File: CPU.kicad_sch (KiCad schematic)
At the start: 153 parts, among them P1 Conn_02x36_Top_Bottom, P2 Conn_02x13_Top_Bottom, P3 Conn_02x13_Top_Bottom, P4 Conn_02x08_Counter_Clockwise, P5 Conn_02x25_Counter_Clockwise, P6 Conn_02x25_Counter_Clockwise, P7 Conn_02x07_Counter_Clockwise

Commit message: partial memory board
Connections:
- net Sys.PA_{14} is gone; now on net Sys.~{PA_{14}}: P1.19 (Pin_19)
- net Sys.~{Parity}: now reaches P1.29 (Pin_29), U_A13.11
- net Sys.~{INTACK}: now reaches P1.65 (Pin_65), U_A14.11
- net Sys.~{PA_{14}}: now reaches U_A9.12 (BUS2)
- net A13D_a renamed ParitySelect
- net DMA_P2_12 renamed DMAINTRequest
- net E10_8_F14_2 renamed ~{DMAInterrupt}
- net Sys.A_{0} renamed Sys.~{A_{0}}
- net Sys.A_{10} renamed Sys.~{A_{10}}
- net Sys.A_{1} renamed Sys.~{A_{1}}
- net Sys.A_{2} renamed Sys.~{A_{2}}
- net Sys.A_{3} renamed Sys.~{A_{3}}
- net Sys.A_{4} renamed Sys.~{A_{4}}
- net Sys.A_{5} renamed Sys.~{A_{5}}
- net Sys.A_{6} renamed Sys.~{A_{6}}
- net Sys.A_{7} renamed Sys.~{A_{7}}
- net Sys.A_{8} renamed Sys.~{A_{8}}
- net Sys.A_{9} renamed Sys.~{A_{9}}
- net Sys.CA_{15} renamed Sys.~{CA_{15}}
- net Sys.D_{0} renamed Sys.~{D_{0}}
- net Sys.D_{1} renamed Sys.~{D_{1}}
- net Sys.D_{2} renamed Sys.~{D_{2}}
- net Sys.D_{3} renamed Sys.~{D_{3}}
- net Sys.D_{4} renamed Sys.~{D_{4}}
- net Sys.D_{5} renamed Sys.~{D_{5}}
- net Sys.D_{6} renamed Sys.~{D_{6}}
- net Sys.D_{7} renamed Sys.~{D_{7}}
- net Sys.E_{63} renamed Sys.~{INTREQ}
- net Sys.E_{64} renamed Sys.~{MemFault}
- net Sys.INR0 renamed Sys.~{INR0}
- net Sys.INR1 renamed Sys.~{INR1}
- net Sys.INR2 renamed Sys.~{INR2}
- net Sys.INR3 renamed Sys.~{INR3}
- net Sys.PA_{12} renamed Sys.~{PA_{12}}
- net Sys.PA_{13} renamed Sys.~{PA_{13}}
- net Sys.PA_{15} renamed Sys.~{PA_{15}}
- net Sys.PA_{16} renamed Sys.~{PA_{16}}
- net Sys.PA_{17} renamed Sys.~{PA_{17}}
- net ~{AND_SysE_{64}} renamed MemFault_EN
- net ~{DMA_P2_12} renamed ~{DMAINTRequest}
- net ~{DMA_P2_13} renamed ~{DMARequest}
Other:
- note added: "F14D = LOW IF (SW_H=open AND DMA Interrupt) typically HIGH"
- note added: "Sys.~{INR3}"
- note removed: "BusCtl Func: DMA?"
- note removed: "F14D = LOW IF (SW_H=open AND DMA_INT_Request?) typically HIGH"
- note removed: "INT ACK ?"
- moved on the sheet: U_A13D, U_A14D

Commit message: lots of layout and DMA labels, weeee
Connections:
- net MW.D3_{3} is gone; now on net TODO_D3_{3}: U_L5.9 (Q3)
- net SEQ.S_{0} is gone; now on net SEQ.SH_{0}: U_J7.16 (S_{0}), U_L9.10 (S_{0})
- net ~{H14_OE} is gone; now on net TODO_A8_7: U_D5.12 (Q4), U_H14.1 (OEa)
- net DataF.D_{0}: now also U_K7.5 (R_{0})
- net DataF.D_{1}: now also U_K7.4 (R_{1})
- net DataF.D_{2}: now also U_K7.3 (R_{2})
- net FP.~{ABT}: now also R1.2, U_M14.7 (O1b); no longer P3.16 (Pin_16), R1.1
- net GND: now also DSW1.10, DSW1.11, DSW1.12, DSW1.13, DSW1.14, DSW1.15, DSW1.16, DSW1.9, U_M14.19 (OEb)
- net MW.C4_{0}: now also U_J6.5, U_K6.4
- net MW.F1_{7}: now also U_K9.7 (~{E})
- net ~{DataRDLatch}: now also U_B15.3 (C)
- net DMA.~{StartCycle}: now reaches P2.10 (Pin_10), R4.3 (R2), U_M8.8 (I3a)
- net TODO_D3_{3}: now reaches U_L6.4
- net ~{RTC_INT_Reset}: now reaches U_M13.10 (Q5), U_M9.13 (~{R})
- net DMA.~{AddressControl}: now reaches P2.2 (Pin_2), U_M8.9 (O0b)
- net DMA.~{Enable}: now reaches P2.6 (Pin_6), U_M8.3 (O3b)
- net DMA.~{Enable}: no longer U_M8.16 (O1a)
- net DMA.~{BusWriteOE}: now reaches P2.9 (Pin_9), U_M10.8
- net SEQ.SH_{0}: now reaches U_K6.3
- net AddrHToSys renamed ~{AddrHToSys}
- net C15_~{PE}: no longer names the net of U_B11.6, U_C10.3, U_C15.9 (~{PE}), U_D6.10 (I1c)
- net DMAWrite renamed DMA.Write
- net FPC_P3_9 renamed ~{ResetFlag}
- net J7_S_{1} renamed SEQ.S1_{1}
- net K9_In4 renamed CondRegOrPageOut
- net K9_In5 renamed CondDMARequest
- net K9_In6 renamed CondMemFault
- net K9_In7 renamed CondMultiINT
- net L9_S_{1} renamed SEQ.S2_{1}
- net Sys.~{Parity} renamed Sys.~{ParityTest}
- net ~{DMAINTRequest} renamed DMA.~{INTRequest}
- net ~{DMARequest} renamed DMA.~{Request}
- net ~{FPC_P3_15} renamed ~{FPC_SW_4}
- new net: P3.16 (Pin_16), R1.1
- new net DMA.~{End}: U_M8.16 (O1a)
- no-connect marks 54 -> 60
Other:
- note added: "(IN)"
- note added: "(OUT)"
- note added: "+5"
- note added: "ABT"
- note added: "ABT LED"
- note added: "B8A output goes LOW when all are HIGH: AND PA_{17} AND PA_{16} AND PA_{15}^{(?)} AND PA_{14},PA_{13} AND PA_{11} AND PTR.Q_{7} * ignores PA_{12} * PTR.Q_{7} (high bit) has extra memory functions attached (likely page control and MMIO selection) * this would select (ignoring the page bit): ** 0x3f8nn to 0x3ffnn ** ** 0x3e8nn to 0x3efnn **"
- note added: "Edge Top 11 (aka pin47 or Sys.~{APRE}) is OC and follows the output of B7A (pulls LOW when REGFILE addressed) ~{APRE} is not read by the CPU, it's used by memory/cards"
- note added: "GND"
- note added: "GND?"
- note added: "HALT"
- note added: "Holds at zero while no bus cycle Counts up from zero during a cycle Stops at 15 and asserts Sys.~{DRDY}"
- note added: "INR is not in order"
- note added: "Line Clock"
- note added: "MAP0"
- note added: "MAP1"
- note added: "MAP2"
- note added: "RUN"
- note added: "RUN/~{HALT}"
- note added: "SS 2 (OPSYS)"
- note added: "SS 4 (R/F)"
- note added: "SW_M SW_O probably need pull R"
- note added: "SW_O"
- note added: "See E6 (K12.4?)"
- note added: "SysCtl.0 DMA"
- note added: "SysCtl.1 DMA"
- note added: "TODO M8.3,16 to P2"
- note added: "This loads the Condition Register (through extra logic?)"
- note added: "Write/~{Read}"
- note added: "these 3 pins drive the register file index their order does not matter after this point"
- note added: "this half should be GND?"
- note removed: "B8A output goes LOW when all are HIGH: AND PA_{17} AND PA_{16} AND PA_{15}^{(?)} AND PA_{14},PA_{13} AND PA_{11} AND PTR.Q_{7} * ignores PA_{12} * PTR.Q_{7} (high bit) has extra memory functions attached (likely page control and MMIO selection) * this would select (ignoring the high bit): ** 0x3f8nn to 0x3ffnn ** ** 0x3e8nn to 0x3efnn **"
- note removed: "Counts up from zero (sync-load) Stops at 15"
- note removed: "Edge Top 11 (aka pin47 or Sys.~{APRE}) is OC and follows the output of B7A (pulls LOW when REGFILE addressed)"
- note removed: "Sys.~{INR3}"
- note removed: "does M8.12 float? or is the cross connect wrong?"
- note removed: "these three pins drive the register file index their order does not matter after this point"
- moved on the sheet: BODGE1, C39, CR1, P1, P2, P3, P7, R1, R15, R17, R2, R3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

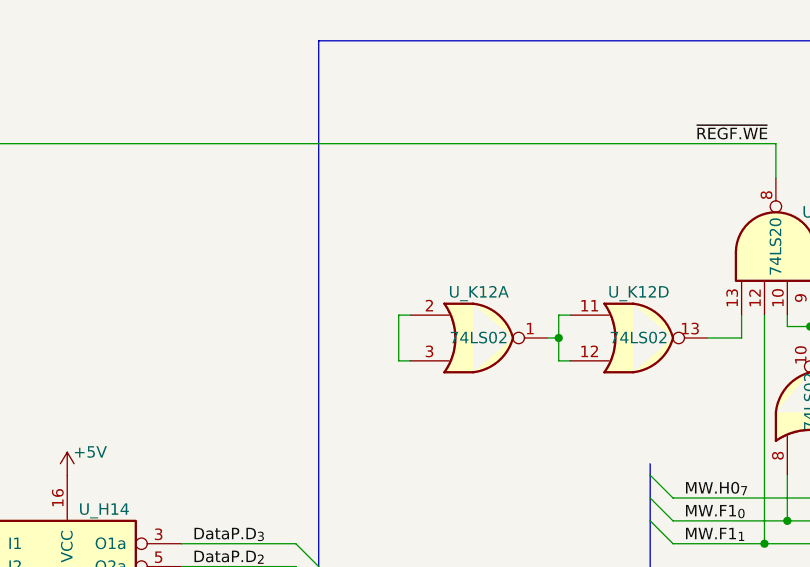
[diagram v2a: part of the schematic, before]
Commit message: an important guess?
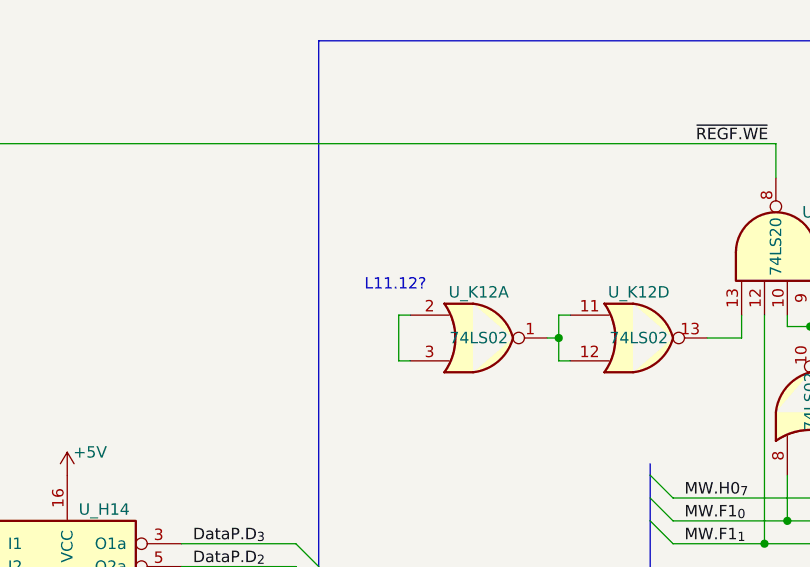
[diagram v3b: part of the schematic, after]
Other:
- note added: "L11.12?"
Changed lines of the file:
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@@
+    (effects (font (size 1.27 1.27)) (justify left bottom))
+  )
+  (text "L11.12?" (at 589.28 114.3 0)
     (effects (font (size 1.27 1.27)) (justify left bottom))
   )

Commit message: all the pins!? and another ERC pass
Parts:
- removed BODGE1: Jumper_2_Bridged, symbol Jumper:Jumper_2_Bridged
- added P10, P8: Conn_02x08_Counter_Clockwise, Package_DIP:DIP-16_W7.62mm_Socket, symbol Connector_Generic:Conn_02x08_Counter_Clockwise
- added unit 3 of U_A1
- added unit 5 of U_A13
- added unit 5 of U_A14
- added unit 7 of U_A15
- added unit 5 of U_A2
- added unit 7 of U_A3
- added unit 4 of U_B11
- added unit 5 of U_B12
- added unit 3 of U_B15
- added unit 2 of U_B7
- added unit 2 of U_B8
- added unit 7 of U_C10
- added unit 5 of U_C7
- added unit 7 of U_C8
- added unit 5 of U_D10
- added unit 5 of U_D12
- added unit 3 of U_D2
- added unit 3 of U_D8
- added unit 4 of U_E10
- added unit 4 of U_E11
- added unit 7 of U_E12
- added unit 7 of U_E14
- added unit 3 of U_E15
- added unit 5 of U_E8
- added unit 3 of U_F12
- added unit 5 of U_F14
- added unit 3 of U_H13
- added unit 7 of U_J6
- added unit 5 of U_K10
- added unit 5 of U_K12
- added unit 5 of U_K6
- added unit 3 of U_L10
- added unit 3 of U_L13
- added unit 5 of U_L14
- added unit 5 of U_L6
- added unit 5 of U_M10
- added unit 3 of U_M9
- C39: footprint (none) -> Capacitor_THT:CP_Axial_L20.0mm_D10.0mm_P26.00mm_Horizontal
- CR1: footprint (none) -> Diode_THT:D_A-405_P10.16mm_Horizontal
- DSW1: footprint (none) -> Package_DIP:DIP-16_W7.62mm_Socket_LongPads
- JP1: footprint (none) -> Connector_PinHeader_2.54mm:PinHeader_1x03_P2.54mm_Vertical
- P1: footprint (none) -> Connector_PCBEdge:BUS_EE200
- P2, P3: footprint (none) -> Connector_IDC:IDC-Header_2x13_P2.54mm_Horizontal
- P4: footprint (none) -> Package_DIP:DIP-16_W7.62mm_Socket
- P5, P6: footprint (none) -> Connector_PinHeader_2.54mm:PinHeader_2x25_P2.54mm_Vertical; symbol Connector_Generic:Conn_02x25_Counter_Clockwise -> Connector_Generic:Conn_02x25_Odd_Even
- P7: footprint (none) -> Package_DIP:DIP-14_W7.62mm_Socket
- R1, R10, R11, R12, R13, R14, R15, R17, R18, R19, R2, R3, R5, R6, R8, R9: footprint (none) -> Resistor_THT:R_Axial_DIN0207_L6.3mm_D2.5mm_P10.16mm_Horizontal
- U_A1, U_A13, U_A14, U_A15, U_A2, U_A3, U_B11, U_B12, U_B15, U_B7, U_B8, U_C10, U_C7, U_C8, U_D10, U_D12, U_D8, U_E10, U_E11, U_E12, U_E14, U_E15, U_E8, U_F12, U_F14, U_H13, U_J6, U_K10, U_K12, U_K6, U_L10, U_L14, U_L6, U_M10, U_M9: footprint (none) -> Package_DIP:DIP-14_W7.62mm
- U_A10, U_A4, U_A5, U_A6, U_A8, U_A9, U_B1, U_B2, U_B3, U_B4, U_B5, U_B6, U_C1, U_C11, U_C12, U_C14, U_C15, U_C2, U_C3, U_C4, U_C5, U_C6, U_D11, U_D2, U_D3, U_D4, U_D5, U_D6, U_D7, U_D9, U_E5, U_E6, U_E7, U_F11, U_F13, U_F6, U_H11, U_H12, U_H14, U_H6, U_J10, U_J11, U_J12, U_J13, U_J9, U_K11, U_K13, U_K9, U_L11, U_L13, U_M12, U_M13: footprint (none) -> Package_DIP:DIP-16_W7.62mm
- U_A11, U_A12, U_A7, U_B13, U_C13, U_C9, U_D13, U_F5, U_H5, U_J5, U_K5, U_L5, U_M14, U_M15, U_M5, U_M6, U_M7, U_M8: footprint (none) -> Package_DIP:DIP-20_W7.62mm
- U_B10, U_B9, U_D14, U_D15: footprint (none) -> Package_DIP:DIP-22_W7.62mm_Socket
- U_J7, U_K7: footprint (none) -> Package_DIP:DIP-28_W15.24mm_Socket
- U_L9: footprint (none) -> Package_DIP:DIP-20_W7.62mm_Socket
- U_MWE2, U_MWF2, U_MWH2, U_MWJ2, U_MWK2, U_MWL2, U_MWM2: footprint (none) -> Package_DIP:DIP-24_W15.24mm_Socket
- XTAL1: footprint (none) -> Crystal:Crystal_HC18-U_Horizontal
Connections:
- net MW.H0_{0} is gone; now on net MWR.H0_{0}: U_D2.2 (A0), U_D3.1 (A0), U_MWE2.9 (Q0)
- net MW.H0_{1} is gone; now on net MWR.H0_{1}: U_D2.3 (A1), U_D3.2 (A1), U_MWE2.10 (Q1)
- net MW.H0_{2} is gone; now on net MWR.H0_{2}: U_D3.3 (A2), U_MWE2.11 (Q2)
- net MW.H0_{3} is gone; now on net MWR.H0_{3}: U_D2.1 (E), U_D3.6 (E3), U_MWE2.13 (Q3)
- net P7_10 is gone; now on net GND: P7.10 (Pin_10)
- net P7_11 is gone; now on net GND: P7.11 (Pin_11)
- net P7_6 is gone; now on net GND: P7.6 (Pin_6)
- net P7_7 is gone; now on net GND: P7.7 (Pin_7)
- net SEQ.PUP is gone; now on net MW.D3_{4}: U_J7.26 (PUSH/~{POP}), U_K7.26 (PUSH/~{POP}), U_L9.20 (PUSH/~{POP})
- net SW_M is gone; now on net Sys.Reset: DSW1.1
- net TODO_M9_1 is gone; now on net ~{Reset_{2}}: U_M9.1 (~{R})
- net TODO_M9_4 is gone; now on net ~{DMAReadEndStrobe}: U_M9.4 (~{S})
- net TODO_VCC is gone; now on net +5V: U_J10.1 (I3)
- net +5V: now also P3.21 (Pin_21), P3.22 (Pin_22), P3.23 (Pin_23), P3.24 (Pin_24), P3.25 (Pin_25), P3.26 (Pin_26), P4.8 (Pin_8), P4.9 (Pin_9), R12.1, R13.1, R15.1, R18.1, R19.1, U_B9.17 (CS2), U_F6.15 (Eb), U_H14.15 (OEb), U_K11.6 (E3), U_K7.23 (C_{n}), U_L13.1 (~{R}), U_L9.3 (~{RE}), U_A1.14 (VCC), U_A13.14 (VCC), U_A14.14 (VCC), U_A15.14 (VCC), U_A2.14 (VCC), U_A3.14 (VCC), U_B11.14 (VCC), U_B12.14 (VCC), U_B15.14 (VCC), U_B7.14 (VCC), U_B8.14 (VCC), U_C10.14 (VCC), U_C7.14 (VCC), U_C8.14 (VCC), U_D10.14 (VCC), U_D12.14 (VCC), U_D2.16 (VCC), U_D8.14 (VCC), U_E10.14 (VCC), U_E11.14 (VCC), U_E12.14 (VCC), U_E14.14 (VCC), U_E15.14 (VCC), U_E8.14 (VCC), U_F12.14 (VCC), U_F14.14 (VCC), U_H13.14 (VCC), U_J6.14 (VCC), U_K10.14 (VCC), U_K12.14 (VCC), U_K6.14 (VCC), U_L10.14 (VCC), U_L13.16 (VCC), U_L14.14 (VCC), U_L6.14 (VCC), U_M10.14 (VCC), U_M9.14 (VCC); no longer R15.2
- net Address.A_{11}: now also P10.16 (Pin_16)
- net Address.A_{12}: now also P10.15 (Pin_15)
- net Address.A_{13}: now also P10.14 (Pin_14)
- net Address.A_{14}: now also P10.13 (Pin_13)
- net Address.A_{15}: now also U_B9.7 (A7), P10.10 (Pin_10), P10.11 (Pin_11), P10.12 (Pin_12)
- net DMA.~{End}: now also P2.5 (Pin_5)
- net DataP.D_{0}: now also U_C11.11 (D3), U_C12.6 (Q3)
- net DataP.D_{3}: now also U_C11.13 (D1), U_C12.4 (Q1)
- net DataP.D_{4}: now also U_C11.6 (Q3), U_C12.11 (D3)
- net DataP.D_{7}: now also U_C11.4 (Q1), U_C12.13 (D1)
- net GND: now also P2.14 (Pin_14), P2.15 (Pin_15), P2.16 (Pin_16), P2.17 (Pin_17), P2.18 (Pin_18), P2.19 (Pin_19), P2.20 (Pin_20), P2.21 (Pin_21), P2.22 (Pin_22), P2.23 (Pin_23), P2.24 (Pin_24), P2.25 (Pin_25), P2.26 (Pin_26), P3.17 (Pin_17), P3.18 (Pin_18), P3.19 (Pin_19), P3.20 (Pin_20), P4.1 (Pin_1), P4.15 (Pin_15), P4.16 (Pin_16), P4.2 (Pin_2), P5.11 (Pin_11), P5.13 (Pin_13), P5.15 (Pin_15), P5.17 (Pin_17), P5.19 (Pin_19), P5.21 (Pin_21), P5.23 (Pin_23), P5.25 (Pin_25), P5.27 (Pin_27), P5.29 (Pin_29), P5.31 (Pin_31), P5.33 (Pin_33), P5.35 (Pin_35), P5.37 (Pin_37), P5.39 (Pin_39), P5.41 (Pin_41), P5.43 (Pin_43), P5.45 (Pin_45), P5.47 (Pin_47), P5.5 (Pin_5), P5.7 (Pin_7), P5.9 (Pin_9), P6.11 (Pin_11), P6.13 (Pin_13), P6.15 (Pin_15), P6.17 (Pin_17), P6.19 (Pin_19), P6.21 (Pin_21), P6.23 (Pin_23), P6.25 (Pin_25), P6.27 (Pin_27), P6.29 (Pin_29), P6.31 (Pin_31), P6.33 (Pin_33), P6.35 (Pin_35), P6.37 (Pin_37), P6.39 (Pin_39), P6.41 (Pin_41), P6.43 (Pin_43), P6.45 (Pin_45), P6.47 (Pin_47), P6.5 (Pin_5), P6.7 (Pin_7), P6.9 (Pin_9), U_A4.9 (OE), U_A5.9 (OE), U_B3.15 (E), U_B4.15 (E), U_B9.19 (~{CS1}), U_C3.15 (E), U_C4.15 (E), U_D11.11 (D3), U_D11.13 (D4), U_D11.14 (D5), U_D9.11 (D3), U_D9.6 (D2), U_E5.4 (D1), U_E5.6 (D2), U_F13.6 (D2), U_F5.1 (~{E}), U_F6.10 (I0b), U_F6.11 (I1b), U_F6.12 (I2b), U_F6.13 (I3b), U_H5.1 (~{E}), U_J12.1 (Ea), U_J12.15 (Eb), U_J5.1 (~{E}), U_J7.10 (OR_{1}), U_J7.12 (OR_{0}), U_J7.6 (OR_{3}), U_J7.8 (OR_{2}), U_K5.1 (~{E}), U_L13.2 (J), U_L5.1 (~{E}), U_M12.13 (D4), U_M12.14 (D5), U_M15.1 (OEa), U_M15.19 (OEb), U_M5.1 (~{E}), U_M8.1 (OEa), U_M8.19 (OEb), U_M9.2 (D), U_MWE2.20 (~{CE_{1}}), U_MWF2.20 (~{CE_{1}}), U_MWH2.20 (~{CE_{1}}), U_MWJ2.20 (~{CE_{1}}), U_MWK2.20 (~{CE_{1}}), U_MWL2.20 (~{CE_{1}}), U_MWM2.20 (~{CE_{1}}), P8.1 (Pin_1), P8.15 (Pin_15), P8.16 (Pin_16), P8.2 (Pin_2), U_A1.7 (GND), U_A13.7 (GND), U_A14.7 (GND), U_A15.7 (GND), U_A2.7 (GND), U_A3.7 (GND), U_B11.7 (GND), U_B12.7 (GND), U_B15.7 (GND), U_B7.7 (GND), U_B8.7 (GND), U_C10.7 (GND), U_C7.7 (GND), U_C8.7 (GND), U_D10.7 (GND), U_D12.7 (GND), U_D2.8 (GND), U_D8.7 (GND), U_E10.7 (GND), U_E11.7 (GND), U_E12.7 (GND), U_E14.7 (GND), U_E15.7 (GND), U_E8.7 (GND), U_F12.7 (GND), U_F14.7 (GND), U_H13.7 (GND), U_J6.7 (GND), U_K10.7 (GND), U_K12.7 (GND), U_K6.7 (GND), U_L10.7 (GND), U_L13.8 (GND), U_L14.7 (GND), U_L6.7 (GND), U_M10.7 (GND), U_M9.7 (GND)
- net MW.F1_{2}: now also U_H11.1 (A0)
- net MW.F1_{3}: now also U_H11.2 (A1)
- net MWS.A_{0}: now also P8.4 (Pin_4)
- net MWS.A_{10}: now also P8.6 (Pin_6)
- net MWS.A_{1}: now also P8.3 (Pin_3)
- net MWS.A_{2}: now also P8.12 (Pin_12)
- net MWS.A_{3}: now also P8.8 (Pin_8)
- net MWS.A_{4}: now also P8.7 (Pin_7)
- net MWS.A_{5}: now also P8.13 (Pin_13)
- net MWS.A_{6}: now also P8.11 (Pin_11)
- net MWS.A_{7}: now also P8.10 (Pin_10)
- net MWS.A_{8}: now also P8.9 (Pin_9)
- net MWS.A_{9}: now also P8.5 (Pin_5)
- net MainClockPhi3: now also U_K12.5
- net P4_7: now also P4.7 (Pin_7)
- net P7_13: now also U_L10.2 (D), U_L10.9 (Q), U_L11.13 (I1d), U_M10.12; no longer DSW1.5, R7.3 (R2), U_M7.2 (I0a)
- net P7_14: now also R11.2, U_MWE2.18 (CE_{3}), U_MWF2.18 (CE_{3}), U_MWH2.18 (CE_{3}), U_MWJ2.18 (CE_{3}), U_MWK2.18 (CE_{3}), U_MWL2.18 (CE_{3}), U_MWM2.18 (CE_{3})
- net PTR.Q_{0}: now also P10.1 (Pin_1)
- net PTR.Q_{2}: now also P10.3 (Pin_3)
- net PTR.Q_{4}: now also P10.5 (Pin_5)
- net PTR.Q_{5}: now also P10.6 (Pin_6)
- net PTR.Q_{6}: now also P10.7 (Pin_7)
- net PTR.~{Q_{7}}: no longer JP1.3 (B), R19.1, U_B12.12
- net VERIFY_CR1: now also R15.2; no longer R15.1
- net ~{ClockB_{1}}: now also U_M12.9 (C)
- net MWR.B5_{4}: now reaches U_F5.13 (D4), U_MWF2.14 (Q4)
- net MWR.B5_{4}: now also P5.20 (Pin_20)
- net MWR.B5_{5}: now reaches U_F5.14 (D5), U_MWF2.15 (Q5)
- net MWR.B5_{5}: now also P5.18 (Pin_18)
- net MWR.B5_{1}: now reaches U_F5.17 (D6), U_MWF2.10 (Q1)
- net MWR.B5_{1}: now also P5.26 (Pin_26)
- net MWR.B5_{0}: now reaches U_F5.18 (D7), U_MWF2.9 (Q0)
- net MWR.B5_{0}: now also P5.28 (Pin_28)
- net MWR.B5_{7}: now reaches U_F5.3 (D0), U_MWF2.17 (Q7)
- net MWR.B5_{7}: now also P5.14 (Pin_14)
- net MWR.B5_{6}: now reaches U_F5.4 (D1), U_MWF2.16 (Q6)
- net MWR.B5_{6}: now also P5.16 (Pin_16)
- net MWR.B5_{2}: now reaches U_F5.7 (D2), U_MWF2.11 (Q2)
- net MWR.B5_{2}: now also P5.24 (Pin_24)
- net MWR.B5_{3}: now reaches U_F5.8 (D3), U_MWF2.13 (Q3)
- net MWR.B5_{3}: now also P5.22 (Pin_22)
- net MWR.D3_{1}: now reaches U_L5.17 (D6), U_MWL2.10 (Q1)
- net MWR.D3_{1}: now also P6.34 (Pin_34)
- net MWR.D3_{2}: now reaches U_L5.7 (D2), U_MWL2.11 (Q2)
- net MWR.D3_{2}: now also P6.32 (Pin_32)
- net MWR.D3_{3}: now reaches U_L5.8 (D3), U_MWL2.13 (Q3)
- net MWR.D3_{3}: now also P6.30 (Pin_30)
- net MWR.D3_{4}: now reaches U_L5.13 (D4), U_MWL2.14 (Q4)
- net MWR.D3_{4}: now also P6.28 (Pin_28)
- net MWR.D3_{5}: now reaches U_L5.14 (D5), U_MWL2.15 (Q5)
- net MWR.D3_{5}: now also P6.26 (Pin_26)
- net MWR.D3_{6}: now reaches U_L5.4 (D1), U_MWL2.16 (Q6)
- net MWR.D3_{6}: now also P6.24 (Pin_24)
- net MWR.D3_{7}: now reaches U_L5.3 (D0), U_MWL2.17 (Q7)
- net MWR.D3_{7}: now also P6.22 (Pin_22)
- net MWR.D3_{0}: now reaches U_L5.18 (D7), U_MWL2.9 (Q0)
- net MWR.D3_{0}: now also P6.36 (Pin_36)
- net MWR.F1_{1}: now reaches U_J5.17 (D6), U_MWJ2.10 (Q1)
- net MWR.F1_{1}: now also P6.2 (Pin_2)
- net MWR.F1_{2}: now reaches U_J5.7 (D2), U_MWJ2.11 (Q2)
- net MWR.F1_{2}: now also P6.1 (Pin_1)
- net MWR.F1_{3}: now reaches U_J5.8 (D3), U_MWJ2.13 (Q3)
- net MWR.F1_{3}: now also P6.3 (Pin_3)
- net MWR.F1_{4}: now reaches U_J5.13 (D4), U_MWJ2.14 (Q4)
- net MWR.F1_{4}: now also P5.49 (Pin_49)
- net MWR.F1_{5}: now reaches U_J5.14 (D5), U_MWJ2.15 (Q5)
- net MWR.F1_{5}: now also P5.50 (Pin_50)
- net MWR.F1_{6}: now reaches U_J5.4 (D1), U_MWJ2.16 (Q6)
- net MWR.F1_{6}: now also P5.48 (Pin_48)
- net MWR.F1_{7}: now reaches U_J5.3 (D0), U_MWJ2.17 (Q7)
- net MWR.F1_{7}: now also P5.46 (Pin_46)
- net MWR.F1_{0}: now reaches U_J5.18 (D7), U_MWJ2.9 (Q0)
- net MWR.F1_{0}: now also P6.4 (Pin_4)
- net at U_K12.2, U_K12.3: now also U_K12.4
- net at R19.2: now also JP1.3 (B), U_B12.12
- net MWR.E2_{1}: now reaches U_M5.17 (D6), U_MWM2.10 (Q1)
- net MWR.E2_{1}: now also P6.50 (Pin_50); no longer P6.26 (Pin_26)
- net MWR.E2_{2}: now reaches U_M5.7 (D2), U_MWM2.11 (Q2)
- net MWR.E2_{2}: now also P6.48 (Pin_48); no longer P6.27 (Pin_27)
- net MWR.E2_{3}: now reaches U_M5.8 (D3), U_MWM2.13 (Q3)
- net MWR.E2_{3}: now also P6.46 (Pin_46); no longer P6.28 (Pin_28)
- net MWR.E2_{4}: now reaches U_M5.13 (D4), U_MWM2.14 (Q4)
- net MWR.E2_{4}: now also P6.44 (Pin_44); no longer P6.29 (Pin_29)
- net MWR.E2_{5}: now reaches U_M5.14 (D5), U_MWM2.15 (Q5)
- net MWR.E2_{5}: now also P6.42 (Pin_42); no longer P6.30 (Pin_30)
- net MWR.E2_{6}: now reaches U_M5.4 (D1), U_MWM2.16 (Q6)
- net MWR.E2_{6}: now also P6.40 (Pin_40); no longer P6.31 (Pin_31)
- net MWR.E2_{7}: now reaches U_M5.3 (D0), U_MWM2.17 (Q7)
- net MWR.E2_{7}: now also P6.38 (Pin_38); no longer P6.32 (Pin_32)
- net MWR.E2_{0}: now reaches U_M5.18 (D7), U_MWM2.9 (Q0)
- net MWR.E2_{0}: now also P6.49 (Pin_49); no longer P6.25 (Pin_25)
- net ~{MainClockPhi3}: now reaches U_H13.13, U_K12.13
- net MWR.H0_{4}: now reaches U_E5.11 (D3), U_MWE2.14 (Q4)
- net MWR.H0_{4}: now also P5.4 (Pin_4)
- net MWR.H0_{6}: now reaches U_E5.13 (D4), U_MWE2.16 (Q6)
- net MWR.H0_{6}: now also P5.1 (Pin_1)
- net MWR.H0_{7}: now reaches U_E5.14 (D5), U_MWE2.17 (Q7)
- net MWR.H0_{7}: now also P5.3 (Pin_3)
- net MWR.H0_{5}: now reaches U_E5.3 (D0), U_MWE2.15 (Q5)
- net MWR.H0_{5}: now also P5.2 (Pin_2)
- net MWR.C4_{4}: now reaches U_H5.13 (D4), U_MWH2.14 (Q4)
- net MWR.C4_{4}: now also P5.36 (Pin_36)
- net MWR.C4_{5}: now reaches U_H5.14 (D5), U_MWH2.15 (Q5)
- net MWR.C4_{5}: now also P5.34 (Pin_34)
- net MWR.C4_{1}: now reaches U_H5.17 (D6), U_MWH2.10 (Q1)
- net MWR.C4_{1}: now also P5.42 (Pin_42)
- net MWR.C4_{0}: now reaches U_H5.18 (D7), U_MWH2.9 (Q0)
- net MWR.C4_{0}: now also P5.44 (Pin_44)
- net MWR.C4_{7}: now reaches U_H5.3 (D0), U_MWH2.17 (Q7)
- net MWR.C4_{7}: now also P5.30 (Pin_30)
- net MWR.C4_{6}: now reaches U_H5.4 (D1), U_MWH2.16 (Q6)
- net MWR.C4_{6}: now also P5.32 (Pin_32)
- net MWR.C4_{2}: now reaches U_H5.7 (D2), U_MWH2.11 (Q2)
- net MWR.C4_{2}: now also P5.40 (Pin_40)
- net MWR.C4_{3}: now reaches U_H5.8 (D3), U_MWH2.13 (Q3)
- net MWR.C4_{3}: now also P5.38 (Pin_38)
- net ~{RT_INT}: now reaches U_F13.15 (Q5), U_H13.1
- net ~{RT_INT}: now also U_M7.8 (I3a)
- net DMA.~{BusReadReady}: now reaches P2.8 (Pin_8), U_M8.18 (O0a)
- net at P1.30 (Pin_30), P1.66 (Pin_66): now also P1.33 (Pin_33), P1.67 (Pin_67), P1.68 (Pin_68), P1.69 (Pin_69)
- net MWR.A6_{4}: now reaches U_K5.13 (D4), U_MWK2.14 (Q4)
- net MWR.A6_{4}: now also P6.12 (Pin_12)
- net MWR.A6_{5}: now reaches U_K5.14 (D5), U_MWK2.15 (Q5)
- net MWR.A6_{5}: now also P6.10 (Pin_10)
- net MWR.A6_{1}: now reaches U_K5.17 (D6), U_MWK2.10 (Q1)
- net MWR.A6_{1}: now also P6.18 (Pin_18)
- net MWR.A6_{0}: now reaches U_K5.18 (D7), U_MWK2.9 (Q0)
- net MWR.A6_{0}: now also P6.20 (Pin_20)
- net MWR.A6_{7}: now reaches U_K5.3 (D0), U_MWK2.17 (Q7)
- net MWR.A6_{7}: now also P6.6 (Pin_6)
- net MWR.A6_{6}: now reaches U_K5.4 (D1), U_MWK2.16 (Q6)
- net MWR.A6_{6}: now also P6.8 (Pin_8)
- net MWR.A6_{2}: now reaches U_K5.7 (D2), U_MWK2.11 (Q2)
- net MWR.A6_{2}: now also P6.16 (Pin_16)
- net MWR.A6_{3}: now reaches U_K5.8 (D3), U_MWK2.13 (Q3)
- net MWR.A6_{3}: now also P6.14 (Pin_14)
- net ~{CCR_EN}: now reaches U_M12.1 (~{E})
- net ~{CCR_EN}: now also U_E6.7 (O7)
- net ~{DMAReadEndStrobe}: now reaches U_B15.11 (C), U_E11.6
- net MWR.H0_{1}: now reaches P5.10 (Pin_10)
- net MWR.H0_{0}: now reaches P5.12 (Pin_12)
- net MWR.H0_{3}: now reaches P5.6 (Pin_6)
- net MWR.H0_{2}: now reaches P5.8 (Pin_8)
- net TODO_J6_4_NC?: now reaches U_J6.4
- net P10_2 renamed PTR.Q_{1}
- net PTR.Q_{1}: now also P10.2 (Pin_2)
- net P10_4 renamed PTR.Q_{3}
- net PTR.Q_{3}: now also P10.4 (Pin_4)
- net P10_8 renamed PTR.Q_{7}
- net PTR.Q_{7}: now also P10.8 (Pin_8)
- net TODO_A6_12 renamed Sys.~{PA_{11}}
- net Sys.~{PA_{11}}: no longer U_A6.12 (BUS2)
- net TODO_A8_7 renamed ~{H14_OE}
- net TODO_B13_16_M13 renamed PROM_Disable
- net TODO_D3_{3} renamed MW.D3_{3}
- net TODO_F7_11_F9_11 renamed ALU.ZERO
- net TODO_H6_2_K5_12 renamed MW.A6_{4}
- net TODO_J12_10_M12_2 renamed CCR.ZERO
- net TODO_J12_11_J9_2 renamed AFL.ZERO
- net TODO_K13_11_F13_12: no longer names the net of U_F13.12 (Q4), U_H13.5, U_K13.11 (I1b)
- net TODO_M12_11_J10: no longer names the net of U_J10.5 (Z), U_M12.11 (D3)
- net TODO_M12_4_J12_7: no longer names the net of U_J12.7 (Za), U_M12.4 (D1)
- net TODO_M12_5_M14 renamed CCR.SIGN
- net TODO_M13_12 renamed INT_ACK
- net TODO_P7_9_R7 renamed TODO_P4
- net TODO_SW_O_8_P3_4 renamed SW_O
- new net SW_R: DSW1.5, R7.3 (R2), U_M7.2 (I0a)
- no-connect marks 60 -> 102
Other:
- note added: "Key Pin"
- note added: "NC"
- note added: "NC?"
- note added: "SW_M"
- note removed: "+5"
- note removed: "GND"
- note removed: "GND?"
- note removed: "L11.12?"
- note removed: "SW_M SW_O probably need pull R"
- note removed: "See E6 (K12.4?)"
- note removed: "TODO"
- note removed: "TODO M8.3,16 to P2"
- note removed: "This loads the Condition Register (through extra logic?)"
- note removed: "needs re-verify pin5/6 is very important here if pin 5, then 1 is VCC if pin 6, then 1 is GND this is needed for SF/RF to work"
- note removed: "this half should be GND?"
- moved on the sheet: R12, R15, R18, R19, U_D2B, U_K12A, U_K12B, U_K12D, U_M10C

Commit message: lots of capacitors, IDC footprints
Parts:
- added C1, C10, C11, C12, C13, C14, C15, C16, C17, C18, C19, C2, C20, C21, C22, C23, C24, C25, C26, C27, C28, C29, C3, C30, C31, C32, C33, C34, C35, C36, C37, C38, C4, C40, C41, C42, C44, C45, C46, C47, C48, C49, C5, C50, C51, C54, C6, C7, C8, C9: 100nF, Capacitor_THT:C_Disc_D4.3mm_W1.9mm_P5.00mm, symbol Device:C_Small
- added C52, C53: 1000uF, Capacitor_THT:CP_Axial_L25.0mm_D10.0mm_P30.00mm_Horizontal, symbol Device:C_Polarized
- C39: value C_Polarized -> 470uF; footprint Capacitor_THT:CP_Axial_L20.0mm_D10.0mm_P26.00mm_Horizontal -> Capacitor_THT:CP_Axial_L18.0mm_D8.0mm_P25.00mm_Horizontal
- P2, P3: symbol Connector_Generic:Conn_02x13_Top_Bottom -> Connector_Generic:Conn_02x13_Odd_Even
- XTAL1: footprint Crystal:Crystal_HC18-U_Horizontal -> Crystal:Crystal_HC52-U_Horizontal
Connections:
- net +5V: now also P3.16 (Pin_16), P3.18 (Pin_18), P3.20 (Pin_20), C1.1, C10.1, C11.1, C12.1, C13.1, C14.1, C15.1, C16.1, C17.1, C18.1, C19.1, C2.1, C20.1, C21.1, C22.1, C23.1, C24.1, C25.1, C26.1, C27.1, C28.1, C29.1, C3.1, C30.1, C31.1, C32.1, C33.1, C34.1, C35.1, C36.1, C37.1, C38.1, C4.1, C40.1, C41.1, C42.1, C44.1, C45.1, C46.1, C47.1, C48.1, C49.1, C5.1, C50.1, C51.1, C52.1, C53.1, C54.1, C6.1, C7.1, C8.1, C9.1; no longer P3.21 (Pin_21), P3.23 (Pin_23), P3.25 (Pin_25)
- net DMA.Write: now also P2.21 (Pin_21); no longer P2.11 (Pin_11)
- net DMA.~{AddressControl}: now also P2.3 (Pin_3); no longer P2.2 (Pin_2)
- net DMA.~{BusReadReady}: now also P2.15 (Pin_15); no longer P2.8 (Pin_8)
- net DMA.~{BusWriteOE}: now also P2.17 (Pin_17); no longer P2.9 (Pin_9)
- net DMA.~{Enable}: now also P2.11 (Pin_11); no longer P2.6 (Pin_6)
- net DMA.~{End}: now also P2.9 (Pin_9); no longer P2.5 (Pin_5)
- net DMA.~{INTRequest}: now also P2.23 (Pin_23); no longer P2.12 (Pin_12)
- net DMA.~{Request}: now also P2.25 (Pin_25); no longer P2.13 (Pin_13)
- net DMA.~{StartCycle}: now also P2.19 (Pin_19); no longer P2.10 (Pin_10)
- net FP.RTI: now also P3.25 (Pin_25); no longer P3.13 (Pin_13)
- net FP.~{RUN}: now also P3.3 (Pin_3); no longer P3.2 (Pin_2)
- net GND: now also P2.10 (Pin_10), P2.12 (Pin_12), P2.2 (Pin_2), P2.4 (Pin_4), P2.6 (Pin_6), P2.8 (Pin_8), P3.10 (Pin_10), P3.12 (Pin_12), P3.14 (Pin_14), P3.8 (Pin_8), C1.2, C10.2, C11.2, C12.2, C13.2, C14.2, C15.2, C16.2, C17.2, C18.2, C19.2, C2.2, C20.2, C21.2, C22.2, C23.2, C24.2, C25.2, C26.2, C27.2, C28.2, C29.2, C3.2, C30.2, C31.2, C32.2, C33.2, C34.2, C35.2, C36.2, C37.2, C38.2, C4.2, C40.2, C41.2, C42.2, C44.2, C45.2, C46.2, C47.2, C48.2, C49.2, C5.2, C50.2, C51.2, C52.2, C53.2, C54.2, C6.2, C7.2, C8.2, C9.2; no longer P2.15 (Pin_15), P2.17 (Pin_17), P2.19 (Pin_19), P2.21 (Pin_21), P2.23 (Pin_23), P2.25 (Pin_25), P3.17 (Pin_17), P3.18 (Pin_18), P3.19 (Pin_19), P3.20 (Pin_20)
- net R4_7: now also P3.4 (Pin_4); no longer P3.15 (Pin_15)
- net SW_2: now also P3.15 (Pin_15); no longer P3.8 (Pin_8)
- net SW_O: now also P3.7 (Pin_7); no longer P3.4 (Pin_4)
- net ~{ResetFlag}: now also P3.17 (Pin_17); no longer P3.9 (Pin_9)
- net at R1.1: now also P3.6 (Pin_6); no longer P3.16 (Pin_16)
- net at U_M15.3 (O3b): now also P3.19 (Pin_19); no longer P3.10 (Pin_10)
- net at P3.11 (Pin_11): now also U_M15.14 (O2a); no longer U_M15.5 (O2b)
- net at U_M15.7 (O1b): now also P3.23 (Pin_23); no longer P3.12 (Pin_12)
- net at U_M15.18 (O0a): now also P3.5 (Pin_5); no longer P3.3 (Pin_3)
- net at U_M15.16 (O1a): now also P3.9 (Pin_9); no longer P3.5 (Pin_5)
- net at U_M15.12 (O3a): now also P3.13 (Pin_13); no longer P3.7 (Pin_7)
- net at U_M8.7 (O1b): now also P2.5 (Pin_5); no longer P2.3 (Pin_3)
- net at U_M8.5 (O2b): now also P2.7 (Pin_7); no longer P2.4 (Pin_4)
- new net: P3.21 (Pin_21), U_M15.5 (O2b)

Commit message: CPU-6 complete?!
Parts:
- added C43: 100nF, Capacitor_THT:C_Disc_D4.3mm_W1.9mm_P5.00mm, symbol Device:C_Small
- DSW1: footprint Package_DIP:DIP-16_W7.62mm_Socket_LongPads -> Button_Switch_THT:SW_DIP_SPSTx08_Slide_9.78x22.5mm_W7.62mm_P2.54mm
- U_F7, U_F9: footprint Package_DIP:DIP-40_W15.24mm -> Package_DIP:DIP-40_W15.24mm_Socket
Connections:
- net TODO_P4 is gone; now on net P7_9: R7.9 (R8), U_L6.9
- net +5V: now also U_D2.15 (E), U_L13.11 (~{S}), U_L13.13 (~{K}), U_L13.15 (~{R}), C43.1
- net GND: now also U_D2.13 (A1), U_D2.14 (A0), U_E12.11, U_E12.13, U_E12.5, U_E12.9, U_E8.8, U_E8.9, U_H14.12 (I5), U_H14.14 (I6), U_J6.3, U_L13.12 (C), U_L13.14 (J), U_L14.1, U_L14.10, U_L14.2, U_L14.9, U_M15.11 (I0b), C43.2
- net MW.C4_{0}: no longer U_J6.3
- net ~{ResetFlag}: now also R4.9 (R8)
- net ~{CPL_Disable}: now reaches P4.14 (Pin_14)
- net ~{CPL_Disable}: now also R13.2, U_E12.1
- net at P2.13 (Pin_13): now also R7.8 (R7)
- net P7_12: no longer names the net of P7.12 (Pin_12)
- net TODO_J6_4_NC?: no longer names the net of U_J6.4
- no-connect marks 102 -> 83
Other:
- note added: "This is needed for ERC"
- note removed: "NC?"
- moved on the sheet: C44, C45, C46, C47, C48, C49, C50, C51, C54, U_D2B, U_E12C, U_E12D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

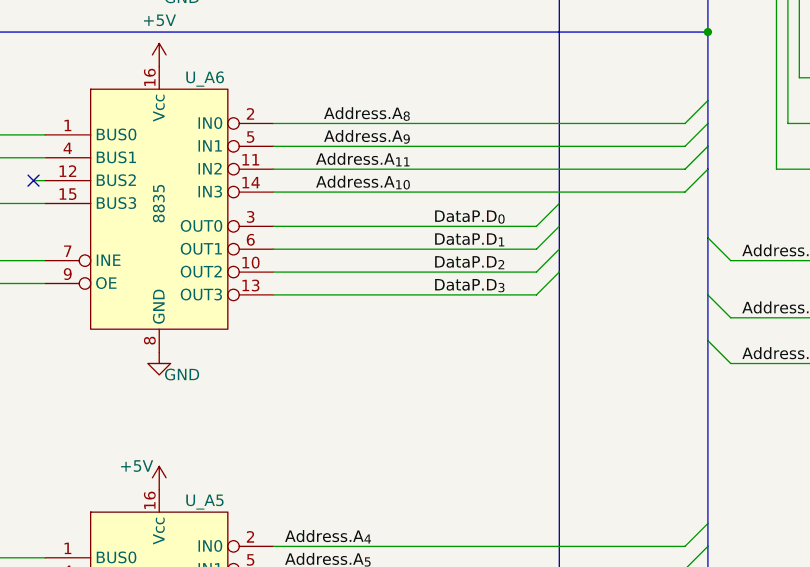
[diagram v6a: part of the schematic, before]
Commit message: small correction
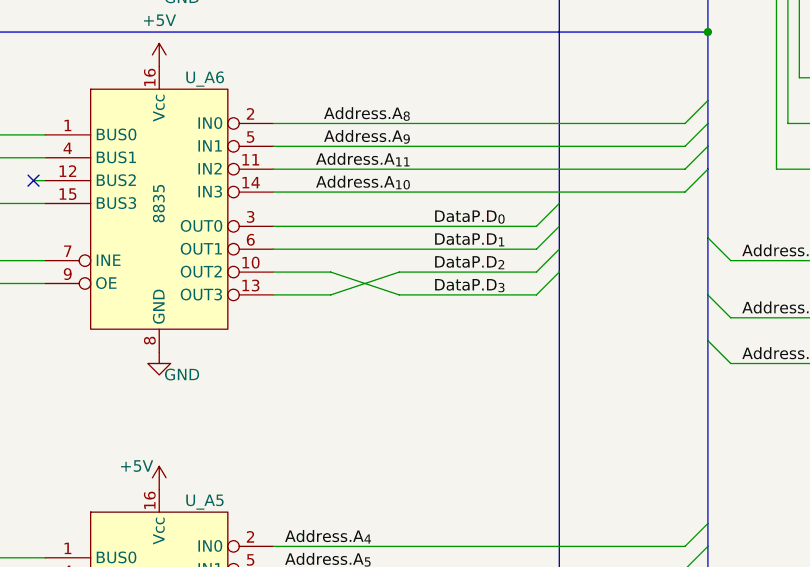
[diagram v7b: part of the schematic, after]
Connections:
- net DataP.D_{2}: now also U_A6.13 (OUT3); no longer U_A6.10 (OUT2)
- net DataP.D_{3}: now also U_A6.10 (OUT2); no longer U_A6.13 (OUT3)
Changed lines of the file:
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@@
     (title "Centurion VI CPU")
     (date "2022-08-02")
-    (rev "24")
+    (rev "25")
     (company "Meisaka Yukara")
     (comment 1 "Visual Reverse Engineered - May contain errors and/or artifacts")
@@
     (stroke (width 0) (type default) (color 0 0 0 0))
   )
+  (wire (pts (xy 143.51 505.46) (xy 151.13 508))
+    (stroke (width 0) (type default) (color 0 0 0 0))
+  )
   (wire (pts (xy 367.03 539.75) (xy 309.88 539.75))
     (stroke (width 0) (type default) (color 0 0 0 0))
@@
     (stroke (width 0) (type default) (color 0 0 0 0))
   )
-  (wire (pts (xy 137.16 505.46) (xy 166.37 505.46))
+  (wire (pts (xy 137.16 505.46) (xy 143.51 505.46))
     (stroke (width 0) (type default) (color 0 0 0 0))
   )
@@
     (stroke (width 0) (type default) (color 0 0 0 0))
   )
+  (wire (pts (xy 143.51 508) (xy 151.13 505.46))
+    (stroke (width 0) (type default) (color 0 0 0 0))
+  )
   (wire (pts (xy 1040.13 444.5) (xy 1042.67 444.5))
     (stroke (width 0) (type default) (color 0 0 0 0))
@@
     (stroke (width 0) (type default) (color 0 0 0 0))
   )
-  (wire (pts (xy 137.16 508) (xy 166.37 508))
+  (wire (pts (xy 137.16 508) (xy 143.51 508))
     (stroke (width 0) (type default) (color 0 0 0 0))
   )
@@
     (stroke (width 0) (type default) (color 0 0 0 0))
   )
+  (wire (pts (xy 151.13 505.46) (xy 166.37 505.46))
+    (stroke (width 0) (type default) (color 0 0 0 0))
+  )
   (wire (pts (xy 598.17 480.06) (xy 637.54 480.06))
     (stroke (width 0) (type default) (color 0 0 0 0))
@@
     (stroke (width 0) (type default) (color 0 0 0 0))
   )
+  (wire (pts (xy 151.13 508) (xy 166.37 508))
+    (stroke (width 0) (type default) (color 0 0 0 0))
+  )
